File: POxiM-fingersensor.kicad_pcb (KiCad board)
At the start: 2 copper layers, 10 x 36.5 mm, 5 parts, among them J3 To readout unit

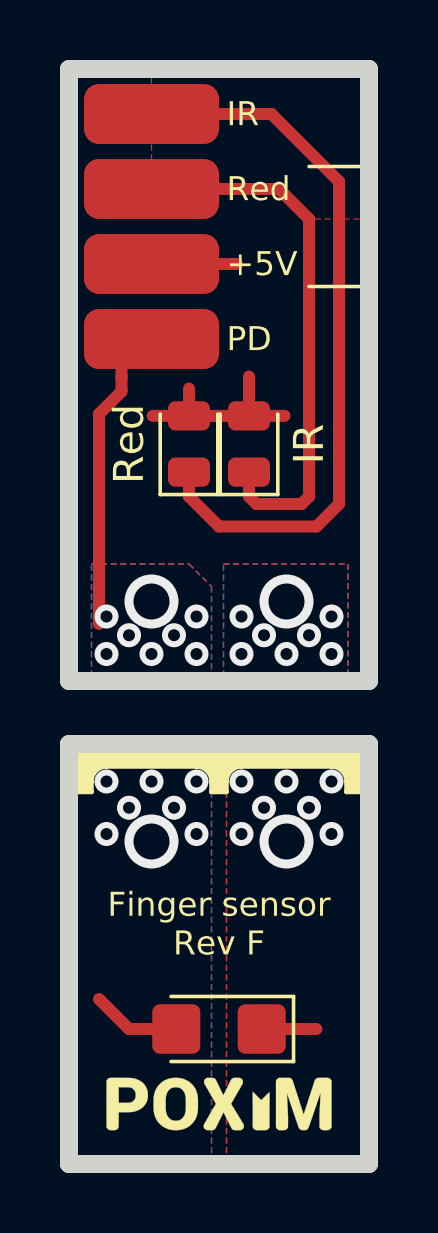
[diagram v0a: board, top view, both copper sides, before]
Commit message: Rev G
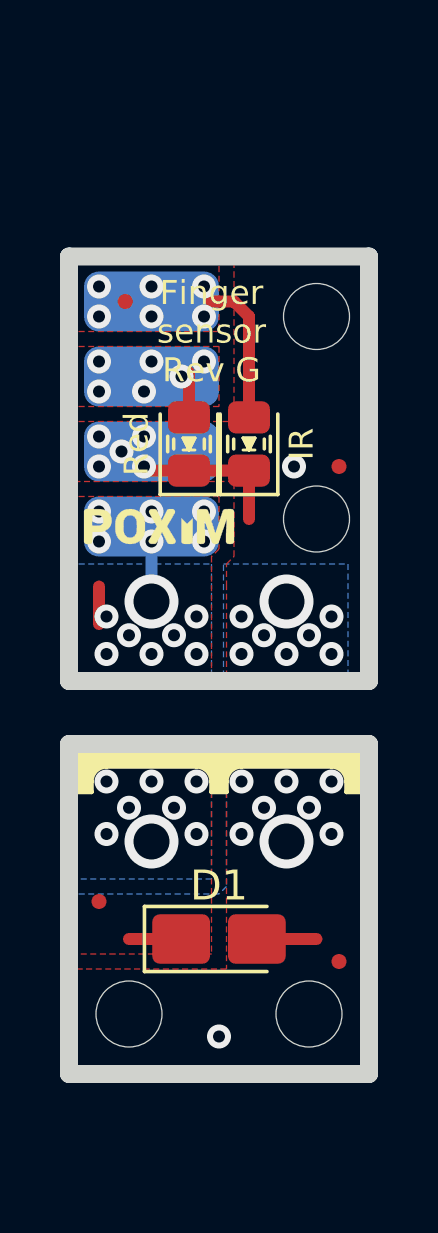
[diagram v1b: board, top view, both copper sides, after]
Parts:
- added FID1: Fiducial, Fiducial:Fiducial_0.5mm_Mask1mm, F.Cu at (105.0, 84.2)
- added FID2: Fiducial, Fiducial:Fiducial_0.5mm_Mask1mm, F.Cu at (113.0, 86.2)
- added FID3: Fiducial, Fiducial:Fiducial_0.5mm_Mask1mm, F.Cu at (105.9, 64.2)
- added FID4: Fiducial, Fiducial:Fiducial_0.5mm_Mask1mm, F.Cu at (113.0, 69.8)
- added G***: LOGO, POxiM-logos:POxiMLogo_GoldHeart_W5mm, F.Cu at (107.0, 71.8)
- added H1: M2 alignment hole, MountingHole:MountingHole_2.2mm_M2, F.Cu at (106.0, 88.0)
- added H2: M2 alignment hole, MountingHole:MountingHole_2.2mm_M2, F.Cu at (112.0, 88.0)
- added H3: M2 alignment hole, MountingHole:MountingHole_2.2mm_M2, F.Cu at (112.2, 64.8)
- added H4: M2 alignment hole, MountingHole:MountingHole_2.2mm_M2, F.Cu at (112.2, 71.5)
- D1: footprint LED_SMD:LED_1206_3216Metric_Castellated -> POxiM-uncategorised:LED_1206_3216Metric_0805_2012Metric_Castellated
- D2, D3: footprint LED_SMD:LED_0805_2012Metric -> POxiM-uncategorised:LED_0805_2012Metric_0603_1608Metric
- G***, J3: moved to B.Cu
- moved J3 6.25 mm to (106.8, 68.0), turned to 180 degrees
- moved G*** 5.75 mm to (109.0, 85.2)
- moved D1 3.00 mm to (109.0, 85.5), turned to 0 degrees
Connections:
- D1 pad 1: +5V -> /Photodiode
- D1 pad 2: /Photodiode -> GND
- D2 pad 1: /LED.IR -> GND
- D2 pad 2: +5V -> /LED.IR
- D3 pad 1: /LED.Red -> GND
- D3 pad 2: +5V -> /LED.Red
- J3 pad 1: /LED.IR -> /LED.Red
- J3 pad 2: /LED.Red -> /LED.IR
- J3 pad 3: +5V -> GND
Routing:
- net /LED.IR: track 24.5 -> 1.58 mm, vias 0 -> 6
- net /LED.Red: track 17.9 -> 4.82 mm, vias 0 -> 6
- net +5V: track 11.3 -> 0.00 mm, vias 16 -> 0
- net /Photodiode: track 12.5 -> 5.33 mm, vias 16 -> 22
- net GND: track 0.00 -> 6.96 mm, vias 0 -> 23
- added copper zone on F.Cu, net /LED.Red
- added copper zone on B.Cu, net GND
- added copper zone on F.Cu, net GND
- removed copper zone on B.Cu, net +5V
- removed copper zone on F.Cu, net +5V
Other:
- board size 10 x 36.5 mm -> 10 x 27.2 mm
- board text added: "Finger sensor Rev G"
- board text added: "GND"
- board text removed: "+5V"
- board text removed: "Finger sensor Rev F"
